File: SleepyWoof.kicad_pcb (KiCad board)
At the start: 2 copper layers, 70.5 x 48 mm, 40 parts, among them J1 Conn_01x04, U1 TLV1704

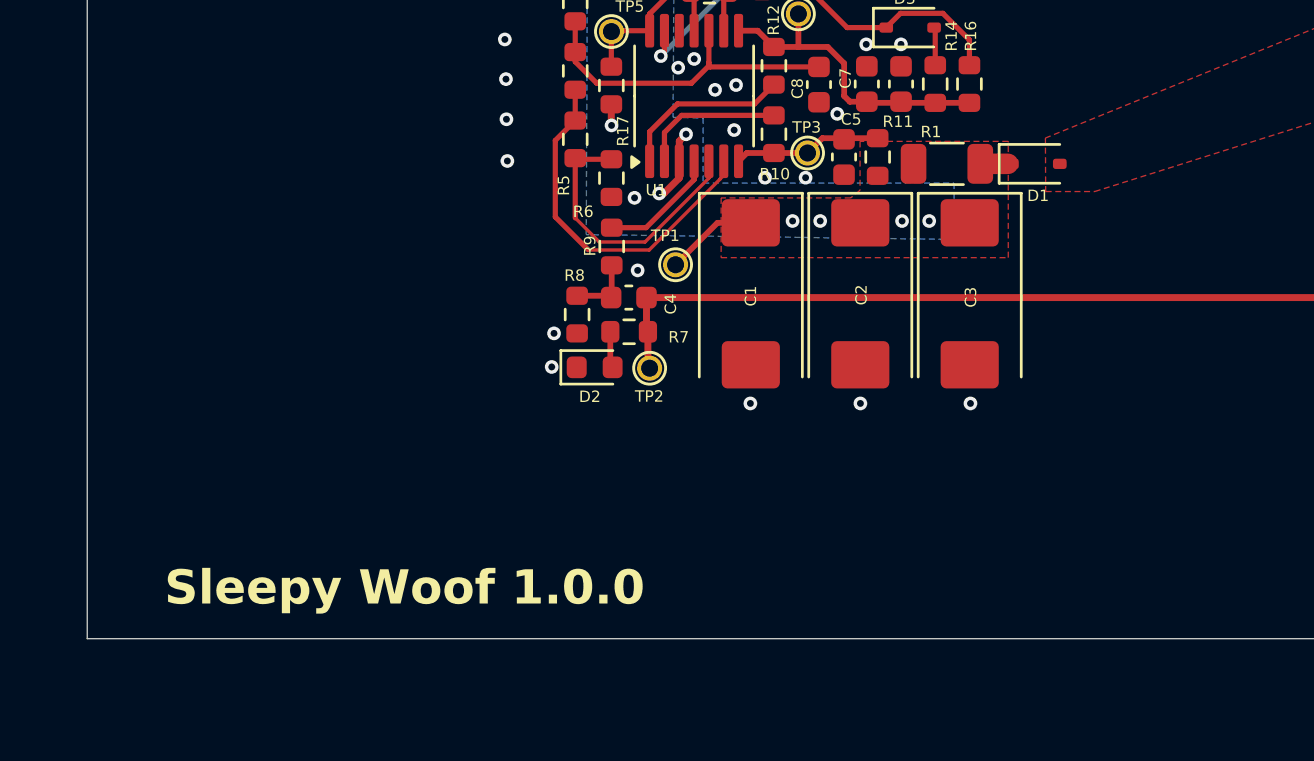
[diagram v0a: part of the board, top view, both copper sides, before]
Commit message: ordered!
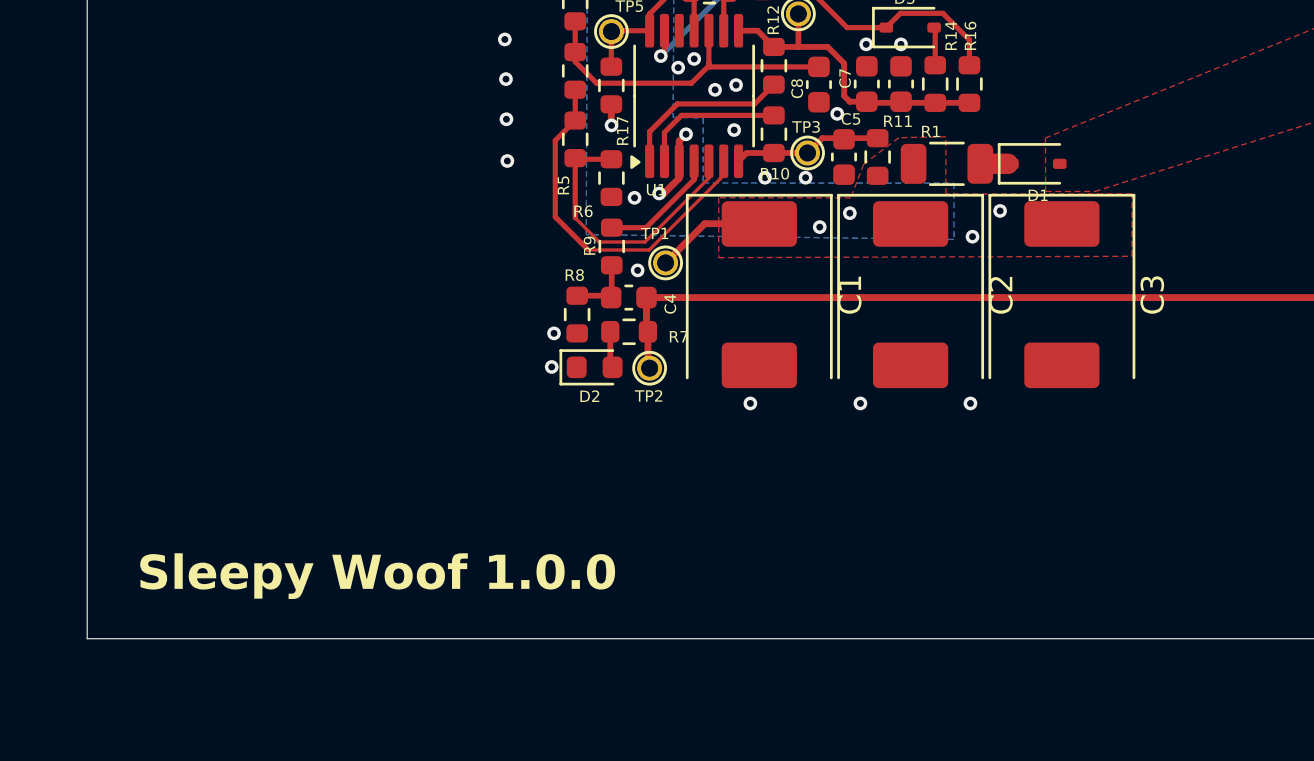
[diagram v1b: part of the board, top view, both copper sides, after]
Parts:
- added G***: LOGO, SleepWoof:sleepy_charlie, B.Cu at (184.2, 101.6)
- C1, C2, C3: footprint Capacitor_Tantalum_SMD:CP_EIA-7343-31_Kemet-D -> Capacitor_Tantalum_SMD:CP_EIA-7361-38_AVX-V
- moved C3 4.04 mm to (188.2, 110.7)
- moved C2 2.21 mm to (181.5, 110.7)
- moved TP1 0.44 mm to (170.8, 109.3)
- moved C1 0.37 mm to (174.9, 110.7)
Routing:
- net /WDT-VIN: track 9.28 -> 10.0 mm
